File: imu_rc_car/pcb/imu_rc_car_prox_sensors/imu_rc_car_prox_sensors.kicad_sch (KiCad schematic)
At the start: 12 parts, among them J1 Conn_01x05_Socket

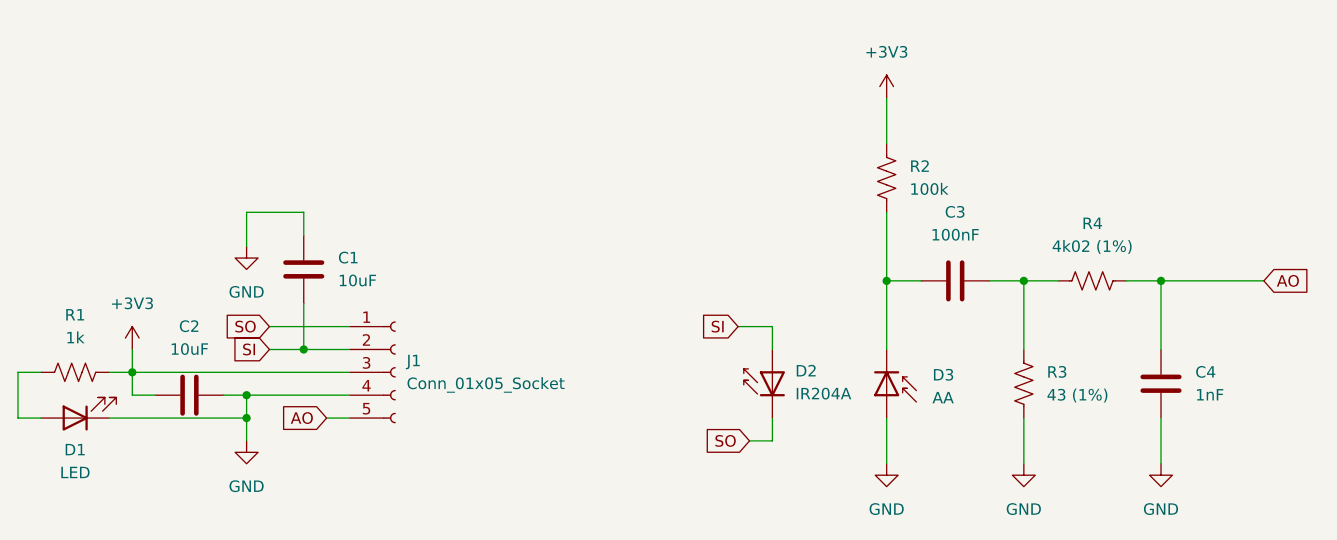
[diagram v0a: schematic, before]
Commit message: commit #27
revision for hand unit complete (board is ready)
board for proximity sensors in series
minor revision in encoder board
progressing work in car board
added essential libraries support for 3D components
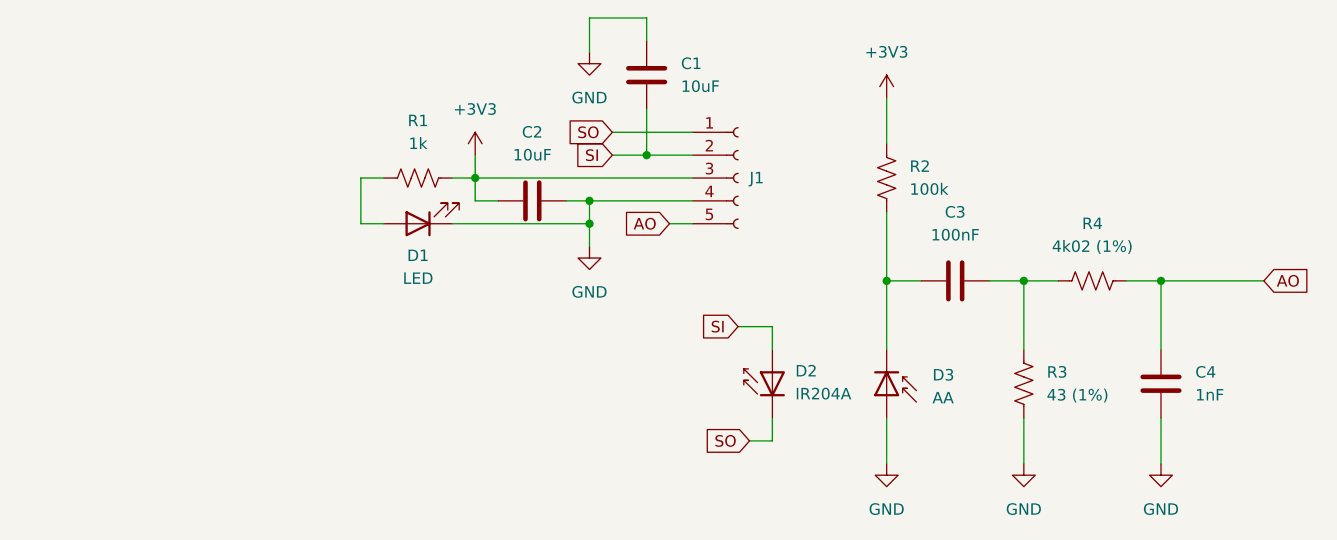
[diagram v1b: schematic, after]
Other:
- moved on the sheet: C1, C2, D1, J1, R1
